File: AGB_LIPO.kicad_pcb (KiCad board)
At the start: 2 copper layers, 49 x 23 mm, 11 parts, among them J1 Conn_01x02_Male, Q1 Si2319CDS, U1 misc_tp4056_board-tp4056, U2 AMS1117-3.3

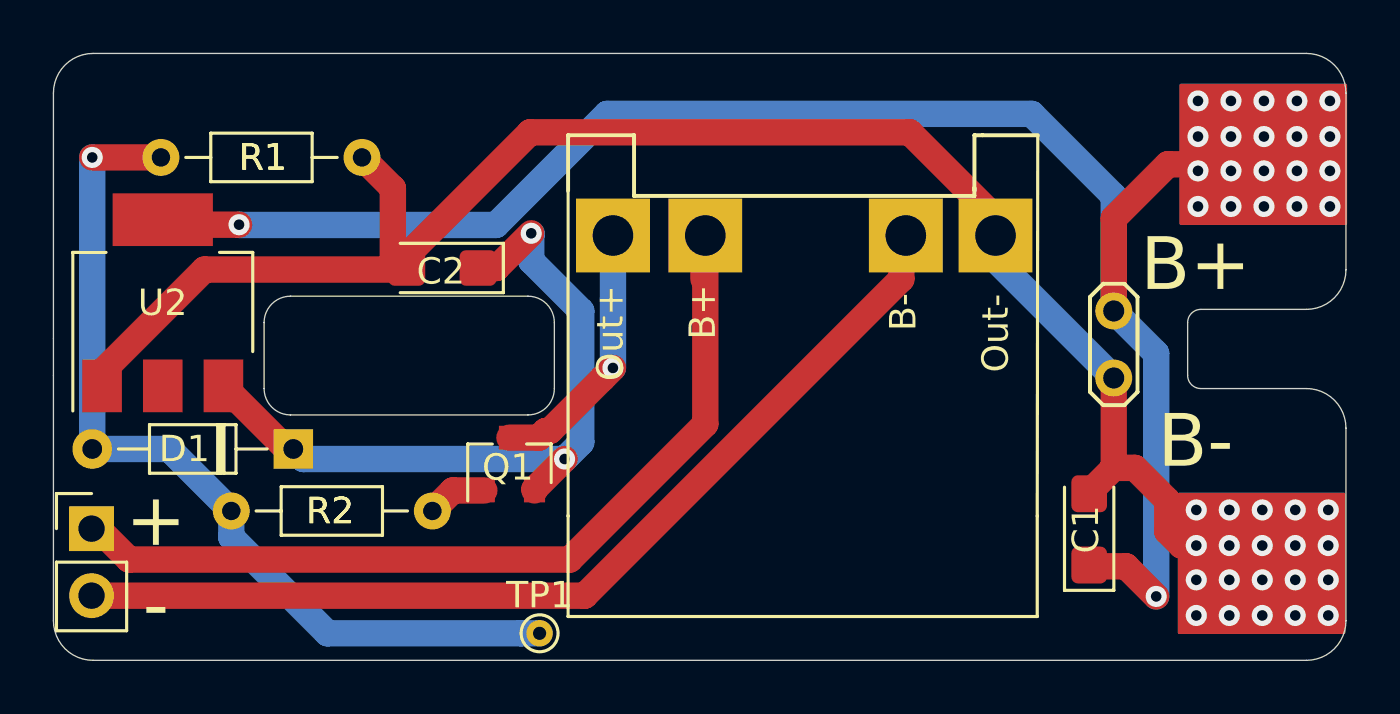
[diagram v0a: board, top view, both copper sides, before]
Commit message: 29/04 Symbol fix
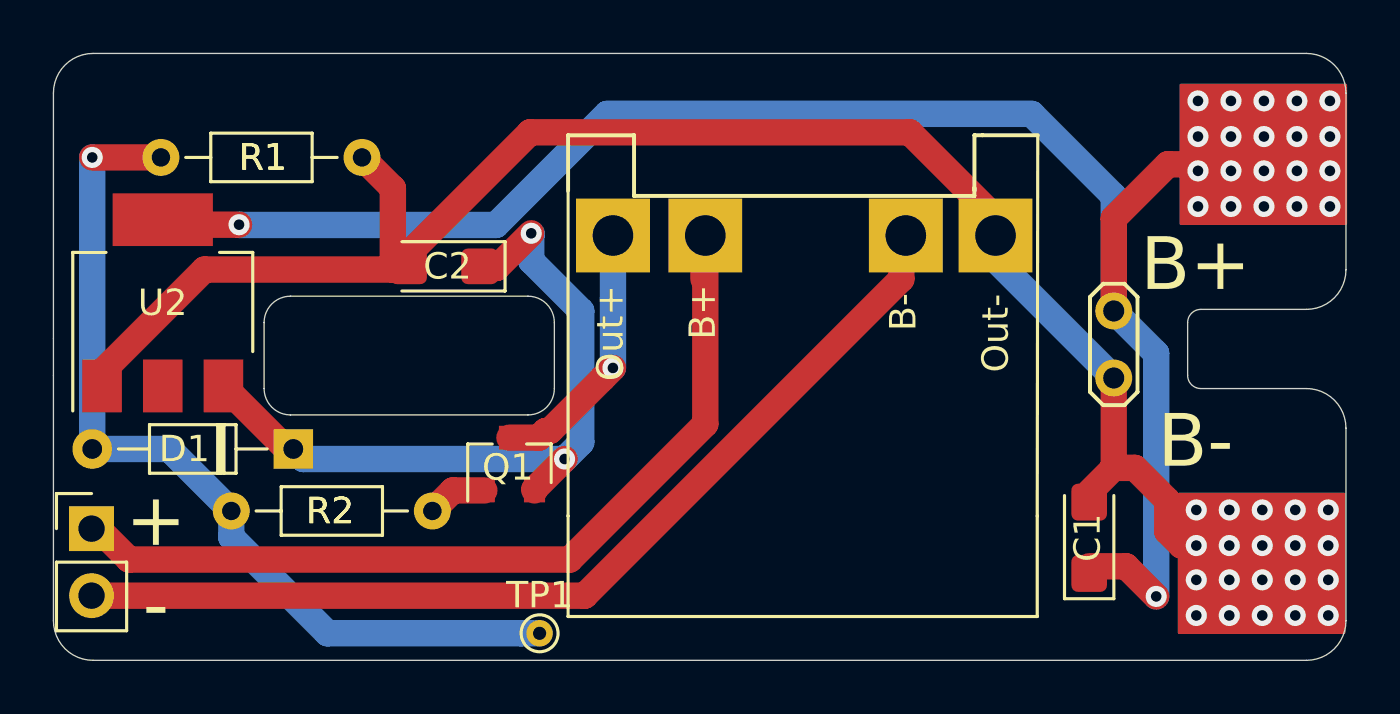
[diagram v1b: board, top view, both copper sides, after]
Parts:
- C2: value C -> 10u
- Q1: value Si2319CDS -> Si2301DS
- moved C1 0.32 mm to (116.3, 37.7)
- moved C2 0.09 mm to (91.8, 27.4)
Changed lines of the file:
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@@
   )
   (module Capacitor_Tantalum_SMD:CP_EIA-3216-18_Kemet-A (layer F.Cu)
-    (at 91.7575 27.432 180)
+    (at 91.821 27.3685 180)
     (descr "Tantalum Capacitor SMD Kemet-A (3216-18 Metric), IPC_7351 nominal, (Body size from: http://www.kemet.com/Lists/ProductCatalog/Attachments/253/KEM_TC101_STD.pdf), generated with kicad-footprint-generator")
     (tags "capacitor tantalum")
     (attr smd)
-    (fp_text reference C2 (at 0.0635 -0.127) (layer F.SilkS)
-      (effects (font (size 1 1) (thickness 0.15)))
-    )
-    (fp_text value C (at 0 1.75) (layer F.Fab)
+    (fp_text reference C2 (at -0.127 0) (layer F.SilkS)
+      (effects (font (size 1 1) (thickness 0.15)))
+    )
+    (fp_text value 10u (at 0 1.75) (layer F.Fab)
       (effects (font (size 1 1) (thickness 0.15)))
     )
@@
   )
   (module Capacitor_Tantalum_SMD:CP_EIA-3216-18_Kemet-A (layer F.Cu)
-    (at 116.2685 37.338 90)
+    (at 116.2685 37.6555 90)
     (descr "Tantalum Capacitor SMD Kemet-A (3216-18 Metric), IPC_7351 nominal, (Body size from: http://www.kemet.com/Lists/ProductCatalog/Attachments/253/KEM_TC101_STD.pdf), generated with kicad-footprint-generator")
     (tags "capacitor tantalum")
     (attr smd)
-    (fp_text reference C1 (at 0 -0.127 90) (layer F.SilkS)
+    (fp_text reference C1 (at 0 -0.0635 90) (layer F.SilkS)
       (effects (font (size 1 1) (thickness 0.15)))
     )
@@
       (effects (font (size 1 1) (thickness 0.15)))
     )
-    (fp_text value Si2319CDS (at 0 2.5 90) (layer F.Fab)
-      (effects (font (size 1 1) (thickness 0.15)))
-    )
+    (fp_text value Si2301DS (at 0 2.5 90) (layer F.Fab)
+      (effects (font (size 1 1) (thickness 0.15)))
+    )

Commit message: Full Circuit redesign
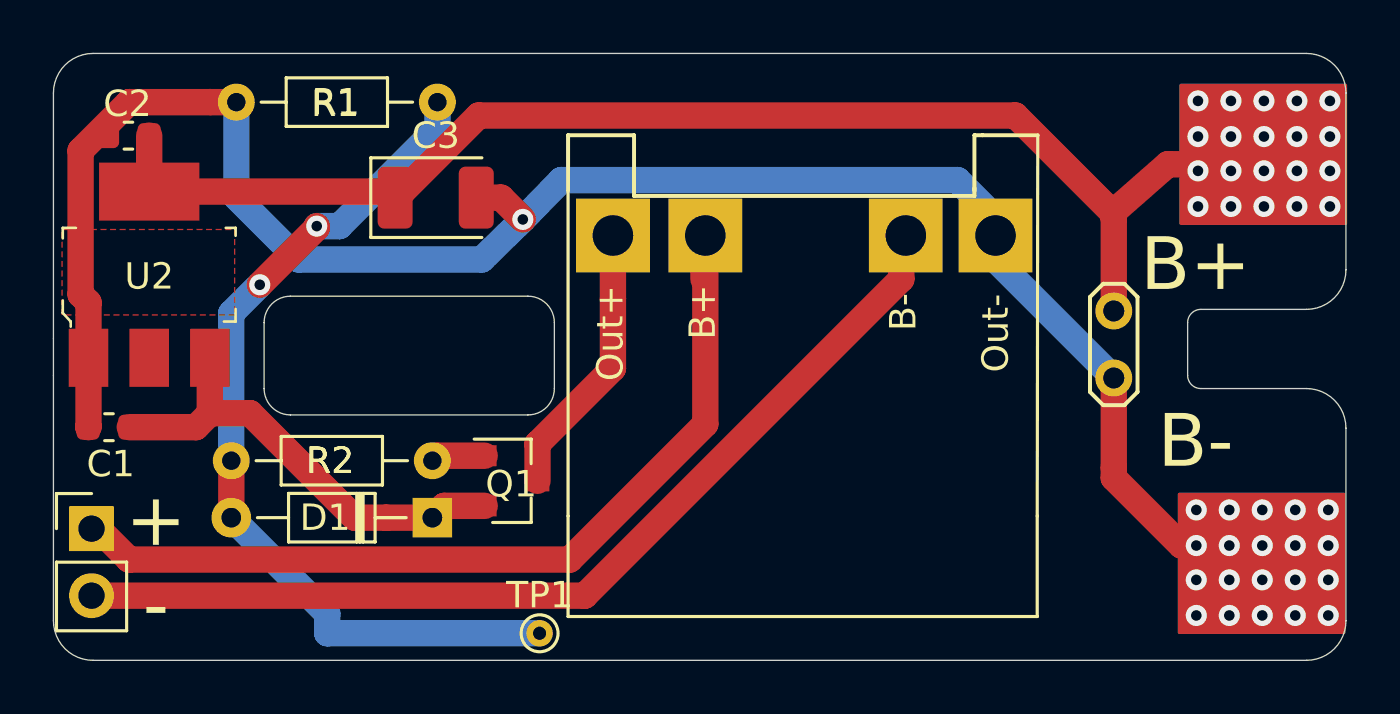
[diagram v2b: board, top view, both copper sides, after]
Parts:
- added C3: 220u, Capacitor_Tantalum_SMD:CP_EIA-3528-21_Kemet-B, F.Cu at (91.5, 24.8)
- C1: value 22u -> 4,7u; footprint Capacitor_Tantalum_SMD:CP_EIA-3216-18_Kemet-A -> Capacitor_SMD:C_0603_1608Metric
- C2: value 10u -> 4,7u; footprint Capacitor_Tantalum_SMD:CP_EIA-3216-18_Kemet-A -> Capacitor_SMD:C_0603_1608Metric
- U2: value AMS1117-3.3 -> AP2114H-3_3TRG1; footprint Package_TO_SOT_SMD:SOT-223-3_TabPin2 -> digikey-footprints:SOT-223
- moved C1 37.4 mm to (79.1, 33.5), turned to 180 degrees
- moved C2 12.9 mm to (79.9, 22.4)
- moved R1 10.7 mm to (91.6, 21.1), turned to 180 degrees
- moved D1 5.88 mm to (91.4, 36.9)
- moved R2 1.91 mm to (83.8, 34.7)
- moved U2 1.18 mm to (80.6, 27.7), turned to 0 degrees
- moved Q1 0.64 mm to (94.4, 35.5), turned to 0 degrees
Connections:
- D1 pad 1: Net-(C2-Pad1) -> Net-(C1-Pad1)
- J1 pad 2: Net-(C1-Pad1) -> Net-(C2-Pad1)
- Q1 pad 2: Net-(C2-Pad1) -> Net-(C1-Pad1)
- U2 pad 2: Net-(C1-Pad1) -> (no net)
- U2 pad 3: Net-(C2-Pad1) -> Net-(C1-Pad1)
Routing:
- net Net-(C1-Pad1): track 67.6 -> 17.6 mm, vias 5 -> 0
- net Net-(C2-Pad1): track 27.9 -> 51.1 mm, vias 2 -> 3
- net Net-(C1-Pad2): track 62.8 -> 71.9 mm, vias 1 -> 2
- net Net-(D1-Pad2): track 34.1 -> 33.4 mm, vias 1 -> 2
- net Net-(Q1-Pad3): track 10.0 -> 10.5 mm, vias 1 -> 0
- added copper zone on F.Cu, net Net-(C1-Pad2)
